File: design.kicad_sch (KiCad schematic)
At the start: 24 parts, among them J1 490107670412, J2 TYPE-C-31-M-12, J4 Conn_02x02_Counter_Clockwise, SW1 5V/3.3V, SW2 D1/D2, SW3 EN, U1 AP2112K-3.3, U2 TCK107AF,LF, U3 CH340C, U4 TS3USB30RSWR

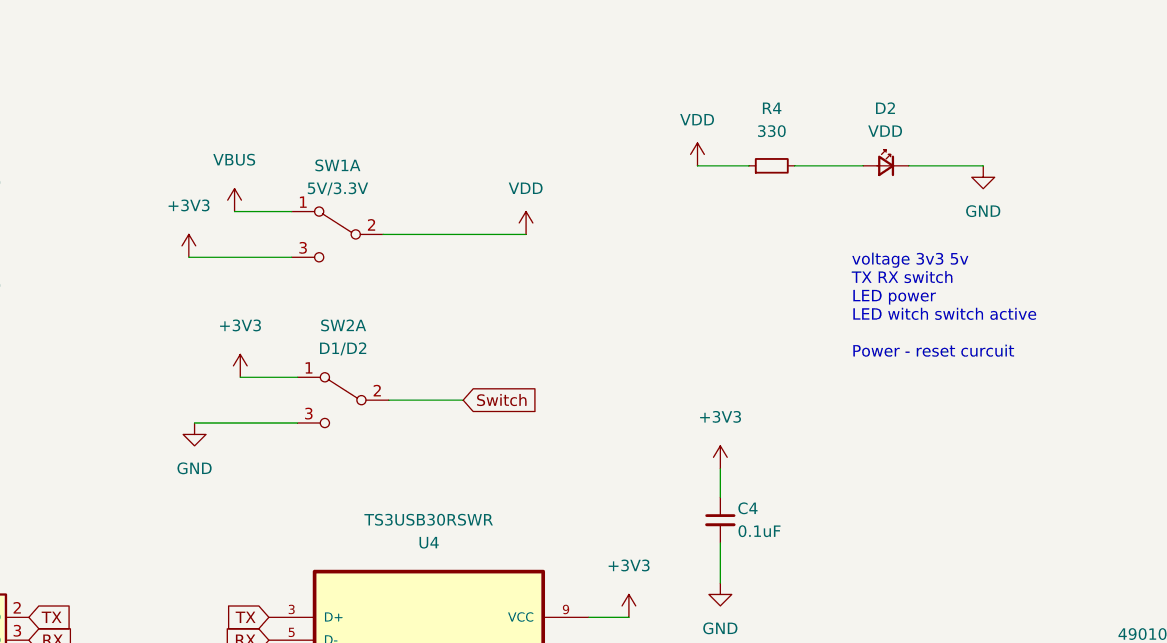
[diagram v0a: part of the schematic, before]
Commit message: update
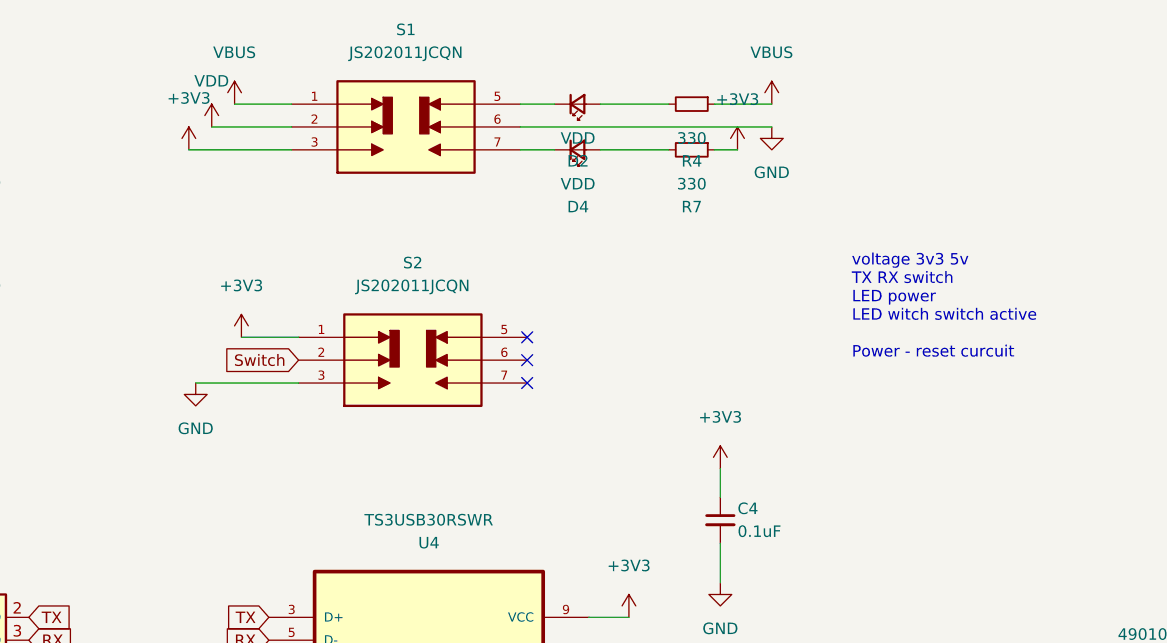
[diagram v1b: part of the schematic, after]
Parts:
- removed SW1: 5V/3.3V, Button_Switch_SMD:SW_DPDT_CK_JS202011JCQN, symbol Switch:SW_DPDT_x2
- removed SW2: D1/D2, Button_Switch_SMD:SW_DPDT_CK_JS202011JCQN, symbol Switch:SW_DPDT_x2
- added D4: VDD, LED_SMD:LED_0805_2012Metric, symbol Device:LED_Small
- added R7: 330, Resistor_SMD:R_0805_2012Metric, symbol Device:R_Small
- added S1, S2: JS202011JCQN, Snapeda:SW_JS202011JCQN, symbol Snapeda:JS202011JCQN
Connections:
- net +3V3: now also R7.1, S1.3, S2.1
- net GND: now also S1.6, S2.3; no longer D2.1 (K)
- net Switch: now also S2.2
- net VBUS: now also R4.1, S1.1
- net VDD: now also S1.2; no longer R4.1
- new net: D4.2 (A), R7.2
- new net: D2.1 (K), S1.5
- new net: D4.1 (K), S1.7
- no-connect marks 9 -> 12

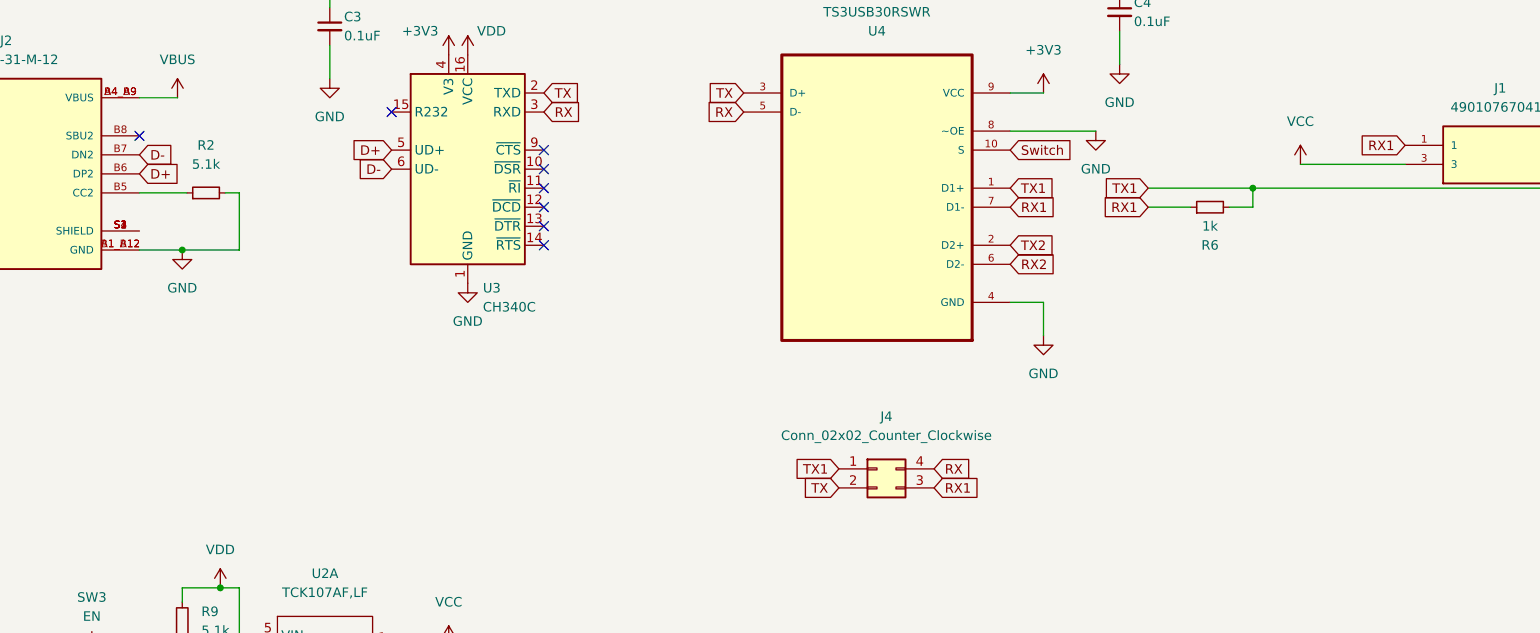
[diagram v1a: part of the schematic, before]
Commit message: update
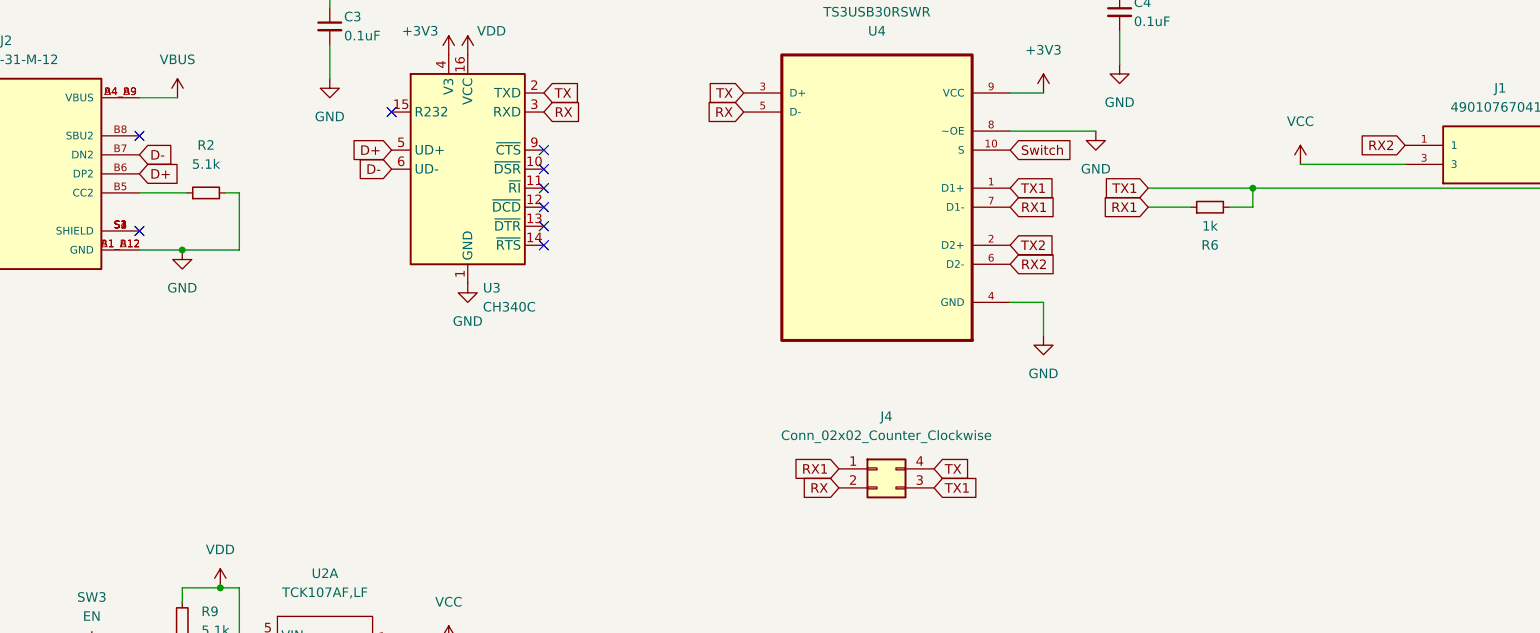
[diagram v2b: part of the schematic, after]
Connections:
- net RX: now also J4.2 (Pin_2); no longer J4.4 (Pin_4)
- net RX1: now also J4.1 (Pin_1); no longer J1.1, J4.3 (Pin_3)
- net RX2: now also J1.1
- net TX: now also J4.4 (Pin_4); no longer J4.2 (Pin_2)
- net TX1: now also J4.3 (Pin_3); no longer J4.1 (Pin_1)
- no-connect marks 12 -> 13
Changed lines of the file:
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@@
   (no_connect (at 27.305 91.44))
   (no_connect (at 62.865 83.82))
+  (no_connect (at 62.865 96.52))
   (no_connect (at 96.52 80.645))
   (no_connect (at 116.84 98.425))
@@
     )
   )
-  (global_label "RX1" (shape input) (at 168.91 130.81 0) (fields_autoplaced)
-    (effects (font (size 1.27 1.27)) (justify left))
-    (property "Referenzen zwischen Schaltplänen" "${INTERSHEET_REFS}" (id 0) (at 174.9232 130.8894 0)
-      (effects (font (size 1.27 1.27)) (justify left) hide)
+  (global_label "RX1" (shape input) (at 156.21 128.27 180) (fields_autoplaced)
+    (effects (font (size 1.27 1.27)) (justify right))
+    (property "Referenzen zwischen Schaltplänen" "${INTERSHEET_REFS}" (id 0) (at 150.1968 128.1906 0)
+      (effects (font (size 1.27 1.27)) (justify right) hide)
     )
   )
@@
     )
   )
-  (global_label "RX" (shape input) (at 168.91 128.27 0) (fields_autoplaced)
-    (effects (font (size 1.27 1.27)) (justify left))
-    (property "Referenzen zwischen Schaltplänen" "${INTERSHEET_REFS}" (id 0) (at 173.7137 128.3494 0)
-      (effects (font (size 1.27 1.27)) (justify left) hide)
+  (global_label "RX" (shape input) (at 156.21 130.81 180) (fields_autoplaced)
+    (effects (font (size 1.27 1.27)) (justify right))
+    (property "Referenzen zwischen Schaltplänen" "${INTERSHEET_REFS}" (id 0) (at 151.4063 130.7306 0)
+      (effects (font (size 1.27 1.27)) (justify right) hide)
     )
   )
@@
     )
   )
-  (global_label "TX" (shape input) (at 156.21 130.81 180) (fields_autoplaced)
-    (effects (font (size 1.27 1.27)) (justify right))
-    (property "Referenzen zwischen Schaltplänen" "${INTERSHEET_REFS}" (id 0) (at 151.7087 130.7306 0)
-      (effects (font (size 1.27 1.27)) (justify right) hide)
+  (global_label "TX" (shape input) (at 168.91 128.27 0) (fields_autoplaced)
+    (effects (font (size 1.27 1.27)) (justify left))
+    (property "Referenzen zwischen Schaltplänen" "${INTERSHEET_REFS}" (id 0) (at 173.4113 128.3494 0)
+      (effects (font (size 1.27 1.27)) (justify left) hide)
     )
   )
@@
     )
   )
-  (global_label "RX1" (shape input) (at 231.775 85.09 180) (fields_autoplaced)
+  (global_label "RX2" (shape input) (at 231.775 85.09 180) (fields_autoplaced)
     (effects (font (size 1.27 1.27)) (justify right))
     (property "Referenzen zwischen Schaltplänen" "${INTERSHEET_REFS}" (id 0) (at 225.7618 85.1694 0)
@@
     )
   )
-  (global_label "TX1" (shape input) (at 156.21 128.27 180) (fields_autoplaced)
-    (effects (font (size 1.27 1.27)) (justify right))
-    (property "Referenzen zwischen Schaltplänen" "${INTERSHEET_REFS}" (id 0) (at 150.4991 128.1906 0)
-      (effects (font (size 1.27 1.27)) (justify right) hide)
+  (global_label "TX1" (shape input) (at 168.91 130.81 0) (fields_autoplaced)
+    (effects (font (size 1.27 1.27)) (justify left))
+    (property "Referenzen zwischen Schaltplänen" "${INTERSHEET_REFS}" (id 0) (at 174.6209 130.8894 0)
+      (effects (font (size 1.27 1.27)) (justify left) hide)
     )
   )
